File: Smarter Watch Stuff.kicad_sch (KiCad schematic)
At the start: 0 parts

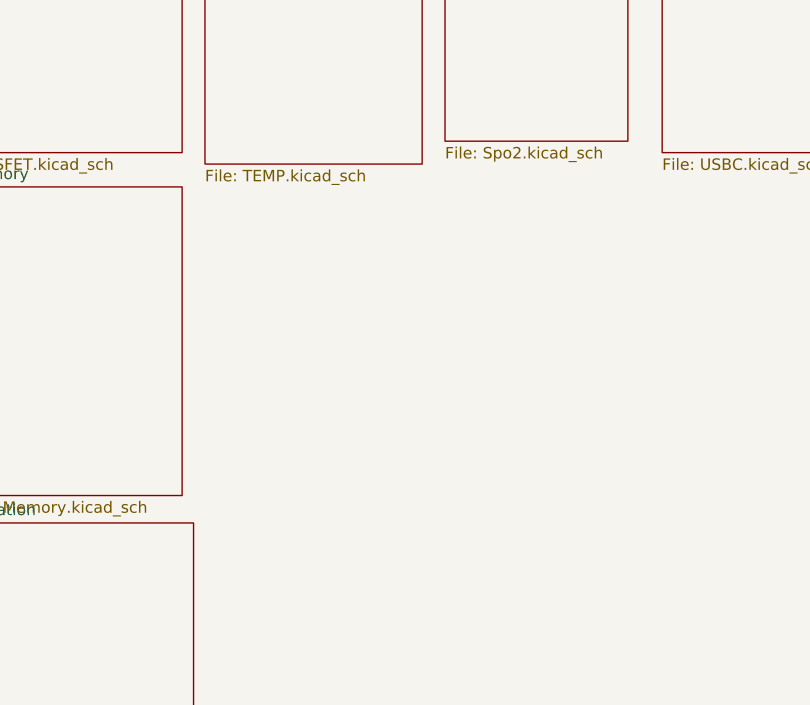
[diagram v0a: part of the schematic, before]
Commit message: ADDED CAP TOUCH
IT OI S GOING TO BE A TOUVHER AND TOUCH U
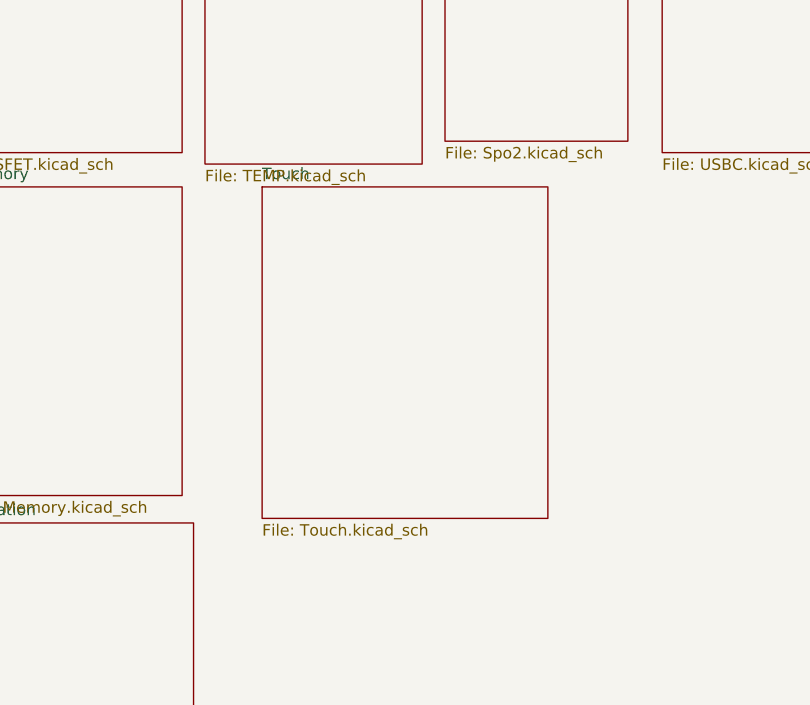
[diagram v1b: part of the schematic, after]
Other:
- added sheet Touch (Touch.kicad_sch)
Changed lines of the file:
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@@
+	)
+	(sheet
+		(at 50.8 90.17)
+		(size 31.75 36.83)
+		(exclude_from_sim no)
+		(in_bom yes)
+		(on_board yes)
+		(dnp no)
+		(fields_autoplaced yes)
+		(stroke
+			(width 0.1524)
+			(type solid)
+		)
+		(fill
+			(color 0 0 0 0.0000)
+		)
+		(property "Sheetname" "Touch"
+			(at 50.8 89.4584 0)
+			(effects
+				(font
+					(size 1.27 1.27)
+				)
+				(justify left bottom)
+			)
+		)
+		(property "Sheetfile" "Touch.kicad_sch"
+			(at 50.8 127.5846 0)
+			(effects
+				(font
+					(size 1.27 1.27)
+				)
+				(justify left top)
+			)
+		)
+		(instances
+			(project "Smarter Watch Stuff"
+				(path "/52181fb0-1be8-41da-83b2-7d5a62778ff4"
+					(page "17")
+				)
+			)
+		)
 	)
 	(sheet
